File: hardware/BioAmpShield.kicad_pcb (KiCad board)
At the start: 2 copper layers, 52.6 x 53.3 mm, 52 parts, among them J1 Conn_01x03, J2 SJ1-3525N, J3 Conn_01x03, J4 Conn_01x02, P1 Power, P2 Analog, P3 Digital, P4 Digital, SW1 SW_Push, SW2 SW_Push, U2 TL074

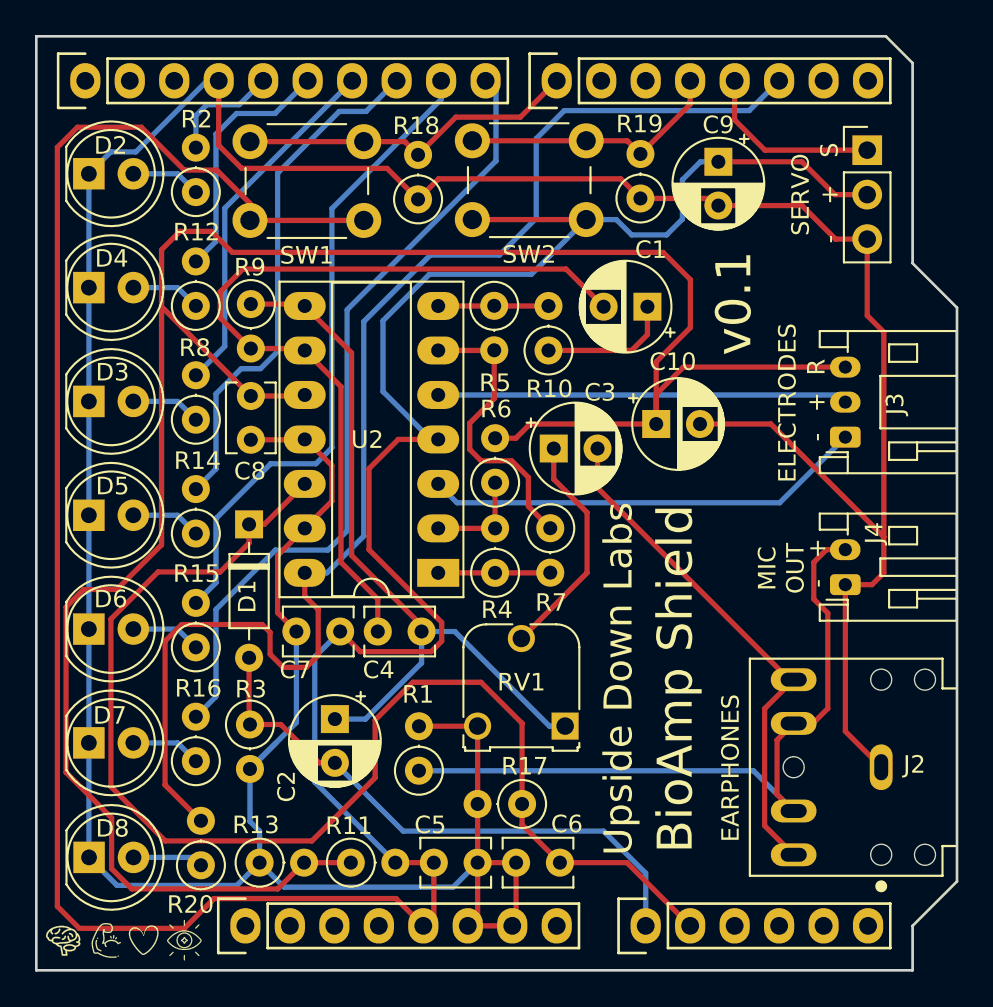
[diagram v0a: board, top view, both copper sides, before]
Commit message: Update information
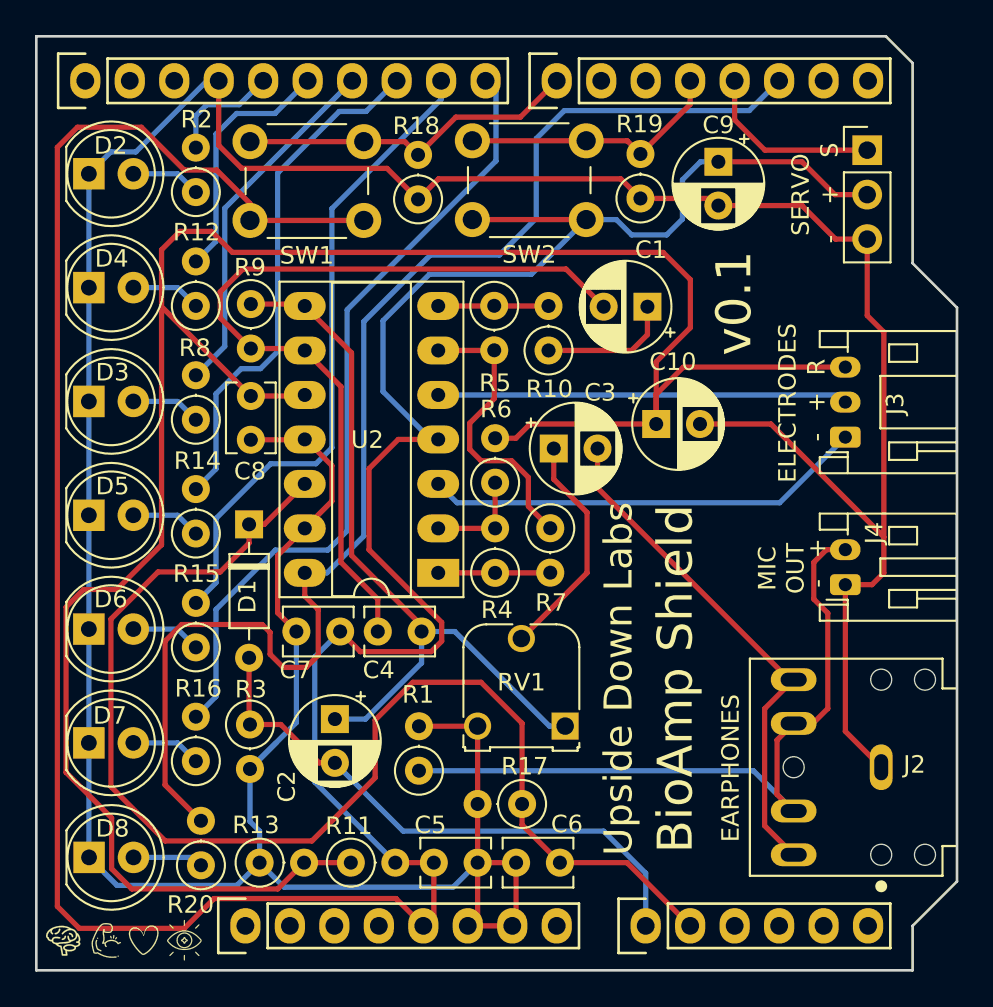
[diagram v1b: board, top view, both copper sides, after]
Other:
- net class Default removed
